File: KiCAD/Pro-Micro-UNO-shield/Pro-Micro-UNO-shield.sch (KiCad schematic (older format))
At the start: 57 parts, among them J1 Arduino_pro_micro, J10 Qwiic I2c, J11 Grove UART, J12 Grove GPIO, J13 SPI header, J14 SPI connector, J15 Debug LED enable, J2 Arduino UNO, J3 Conn_01x10_Male, J4 Conn_01x02_Male, J5 Arduino_pro_micro WIDE, J6 Conn_01x10_Male, J7 Conn_01x02_Male, J9 Grove I2C, SW1 Reset switch

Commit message: Pro micro UNO shield Rev1.1 (Fixed Qwiic connector pin assign)
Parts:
- J10: footprint library:JST_SH_BM04B-SRSS-TB_04x1.00mm_Straight -> library:Qwiic_I2C_1.00mm_4pin
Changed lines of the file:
@@
 F 0 "J10" H 7678 1658 60  0000 L CNN
 F 1 "Qwiic I2c" H 7678 1552 60  0000 L CNN
-F 2 "library:JST_SH_BM04B-SRSS-TB_04x1.00mm_Straight" H 7100 1900 60  0001 C CNN
+F 2 "library:Qwiic_I2C_1.00mm_4pin" H 7100 1900 60  0001 C CNN
 F 3 "" H 7100 1900 60  0001 C CNN
 	1    7100 1900

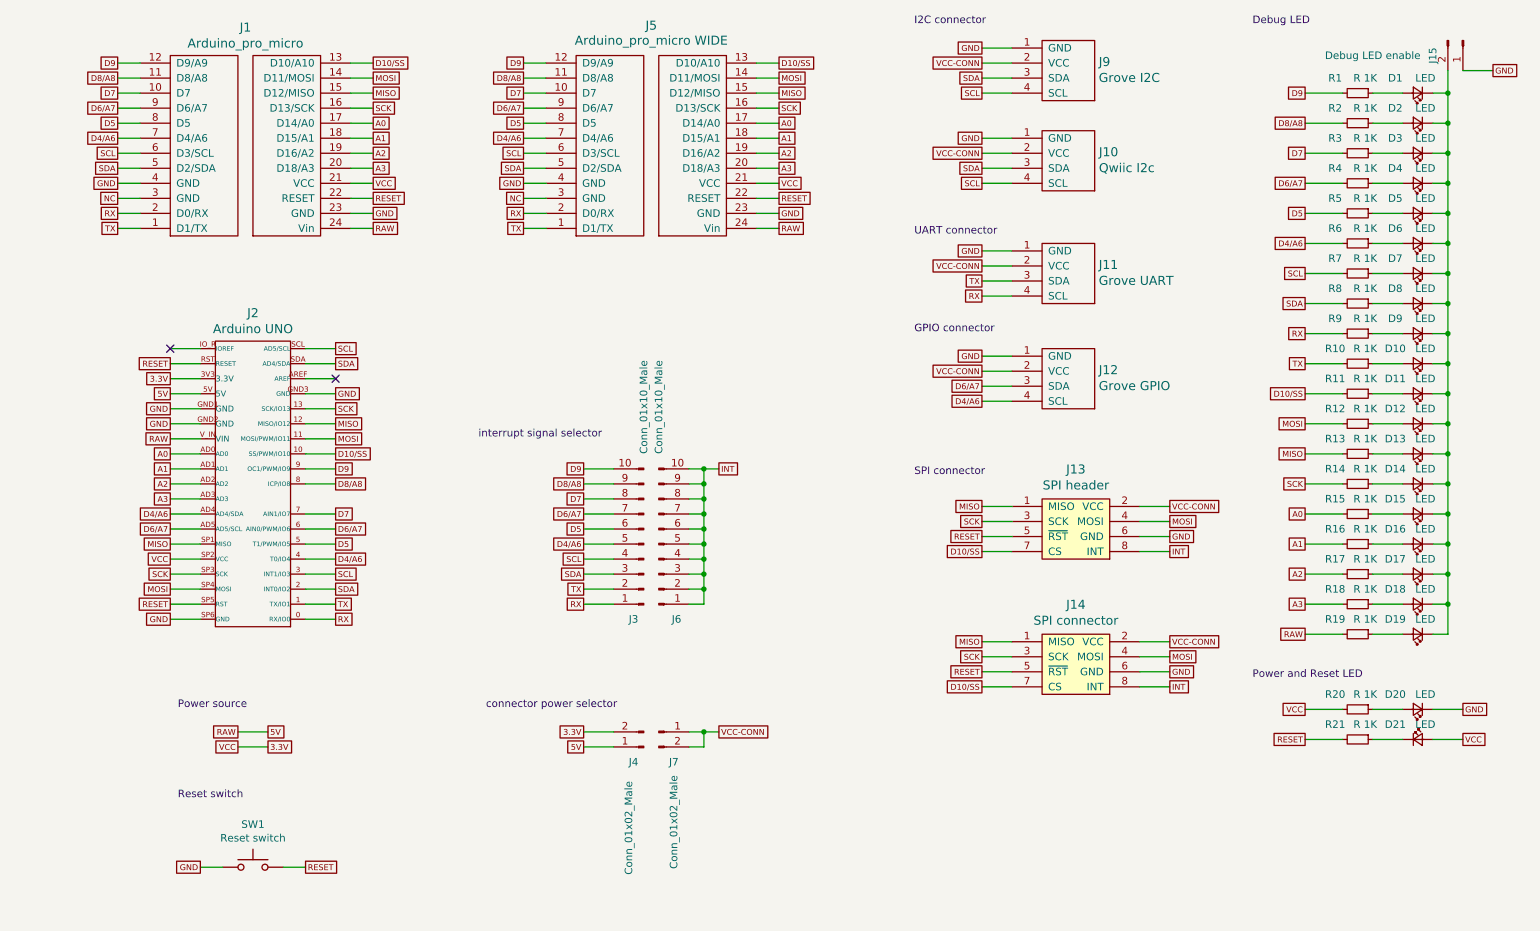
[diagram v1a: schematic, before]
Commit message: Pro Micro UNO shield v2.0 (Diag shield)
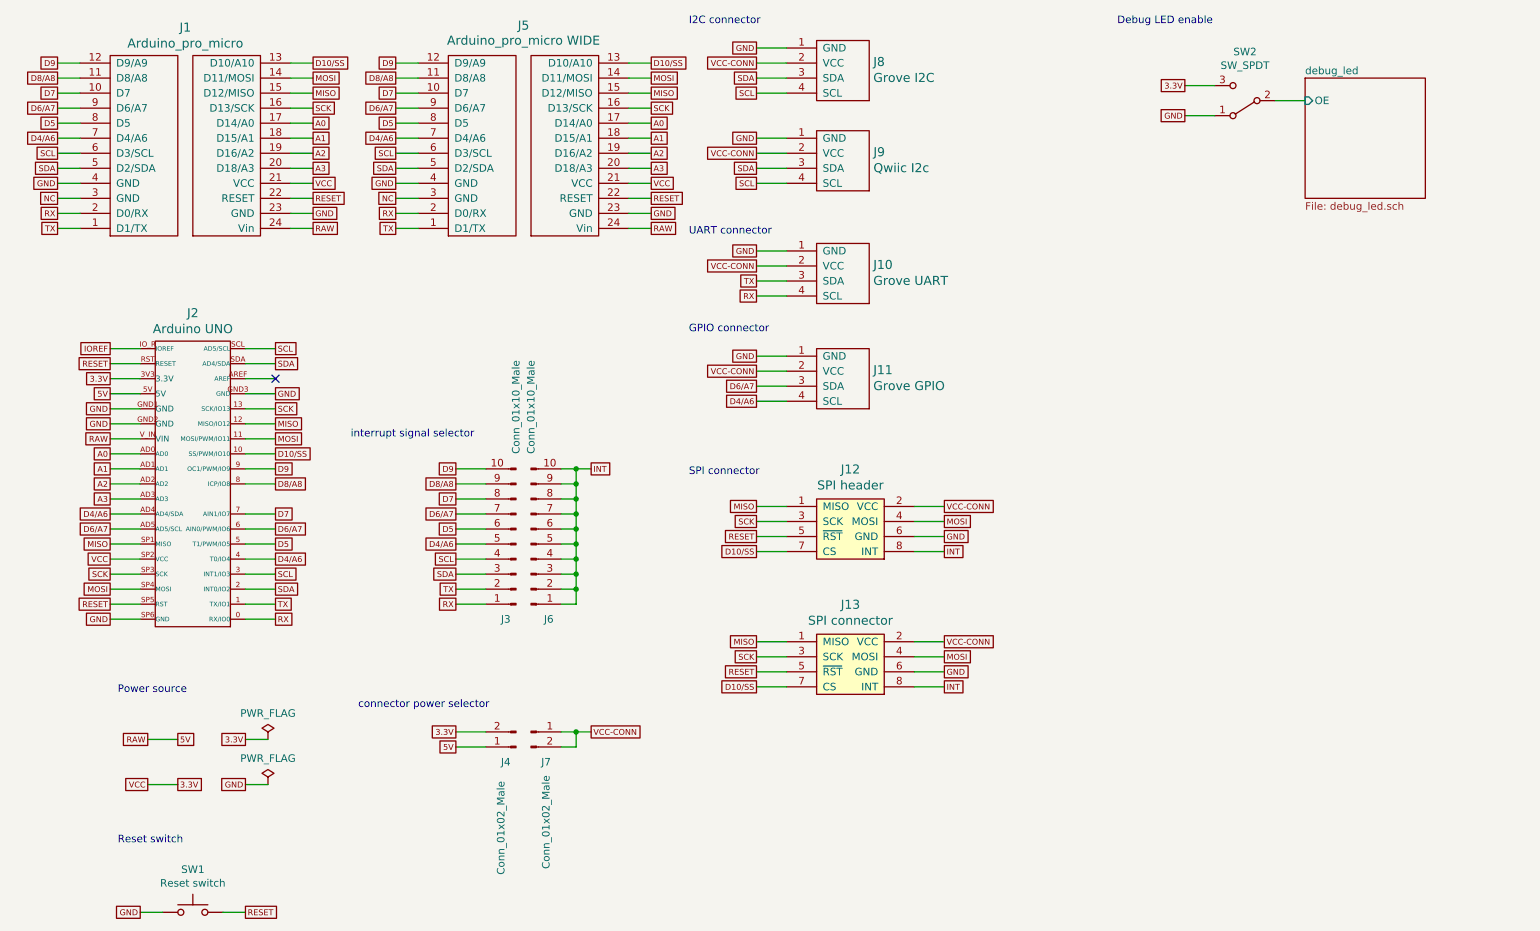
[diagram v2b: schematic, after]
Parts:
- removed D1, D10, D11, D12, D13, D14, D15, D16, D17, D18, D19, D2, D20, D21, D3, D4, D5, D6, D7, D8, D9: LED, KiCAD footprints:LED_0603_1608Metric, symbol Device:LED_Small
- removed J15: Debug LED enable, freetronics_footprints:1X02, symbol Connector:Conn_01x02_Male
- removed R1, R10, R11, R12, R13, R14, R15, R16, R17, R18, R19, R2, R20, R21, R3, R4, R5, R6, R7, R8, R9: R 1K, KiCAD footprints:R_0603_1608Metric, symbol Device:R_Small
- added SW2: SW_SPDT, library:mini_slide_switch, symbol Switch:SW_SPDT
- J12: renamed from J13; footprint KiCAD footprints:PinHeader_2x04_P2.54mm_Vertical -> Connector_PinSocket_2.54mm:PinSocket_2x04_P2.54mm_Vertical
- J3, J6: footprint KiCAD footprints:PinHeader_1x10_P2.54mm_Vertical -> Connector_PinSocket_2.54mm:PinSocket_1x10_P2.54mm_Vertical
- J4, J7: footprint KiCAD footprints:PinHeader_1x02_P2.54mm_Vertical -> Connector_PinSocket_2.54mm:PinSocket_1x02_P2.54mm_Vertical
- renumbered J11 to J10, J12 to J11, J14 to J13, J9 to J8, J10 to J9
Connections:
- net 3.3V: now also SW2.3 (C)
- net GND: now also SW2.1 (A)
- net IOREF: now reaches J2.IO_R (IOREF)
- new net debug_led/OE: SW2.2 (B)
- no-connect marks 2 -> 1
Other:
- note added: "Debug LED enable"
- note removed: "Debug LED"
- note removed: "Power and Reset LED"
- moved on the sheet: J1, J10, J11, J12, J13, J2, J3, J4, J5, J6, J7, J8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
